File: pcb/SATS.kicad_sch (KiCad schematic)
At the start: 36 parts, among them J1 Raspberry_Pi_2_3, J10 SENSE, J11 SENSE Power, J12 EXT_GPIO, J13 EXT_GPIO, J14 EXT_GPIO, J2 A00-432-262-450, J3 AudioJack4_SwitchTR1, J4 5V, J5 3.3V, J6 Card LED, J7 Wiegand, J8 Beep, J9 Card Power, SW1 Main Door Switch, SW2 Serv Door Switch, SW3 Third Reed Switch, U1 MCP23017_SP, U2 MCP23017_SP, U3 CD40109BE, U4 IRLZ14PBF

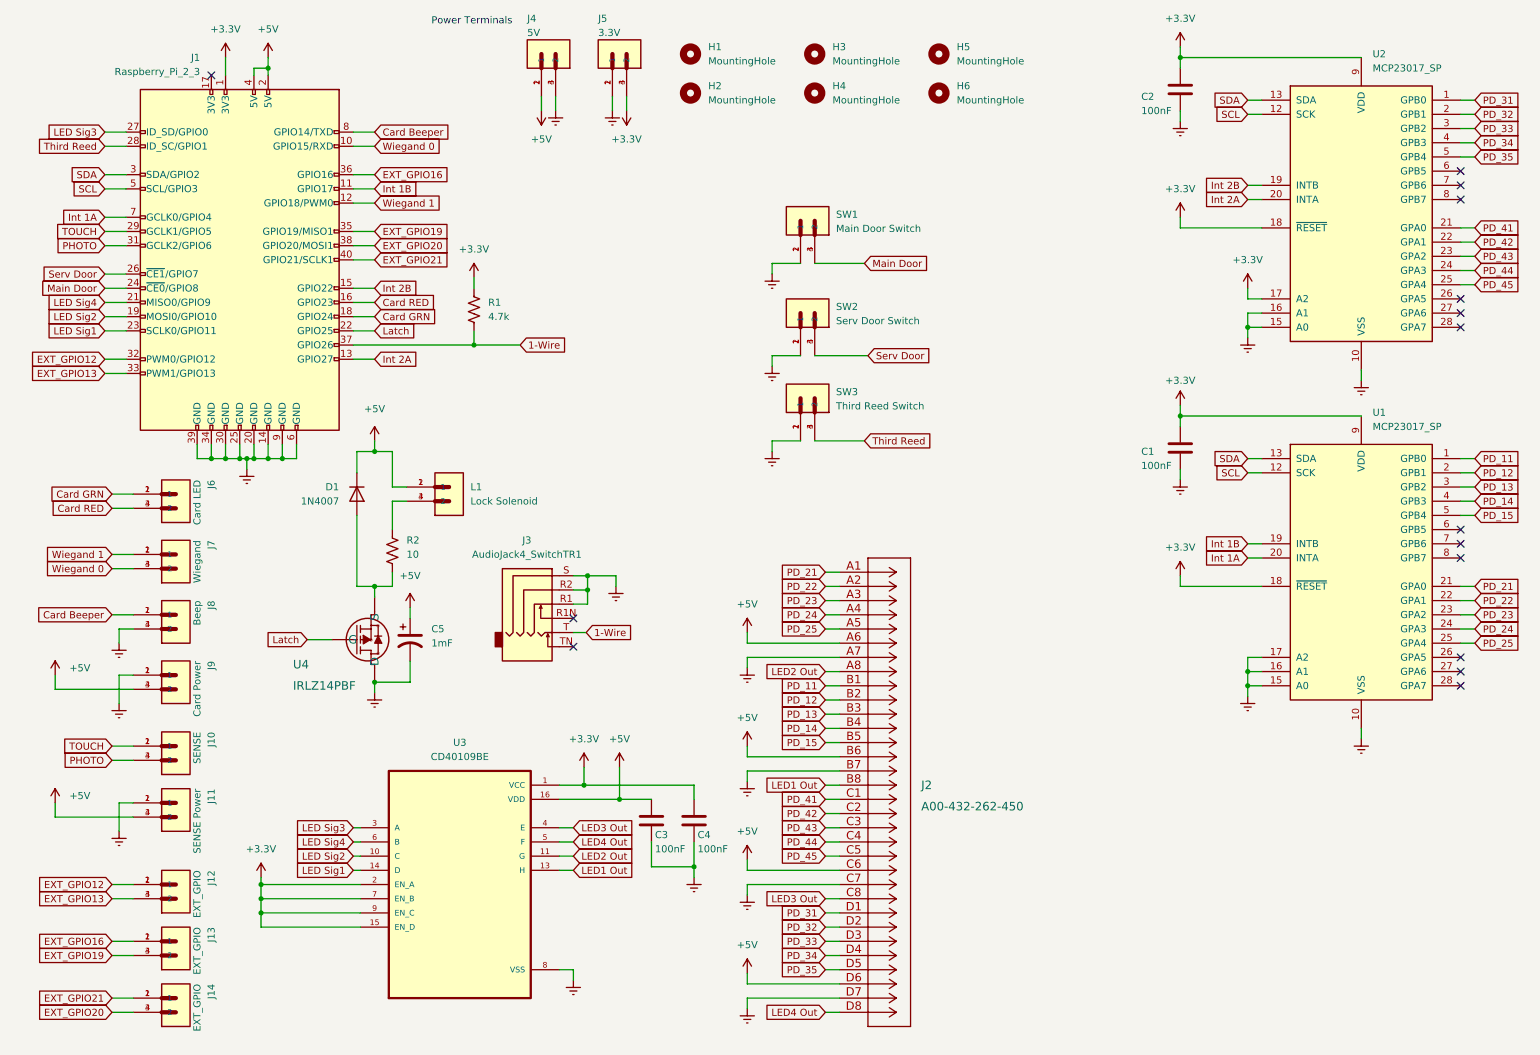
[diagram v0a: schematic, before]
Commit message: Rev 4 - Pretest
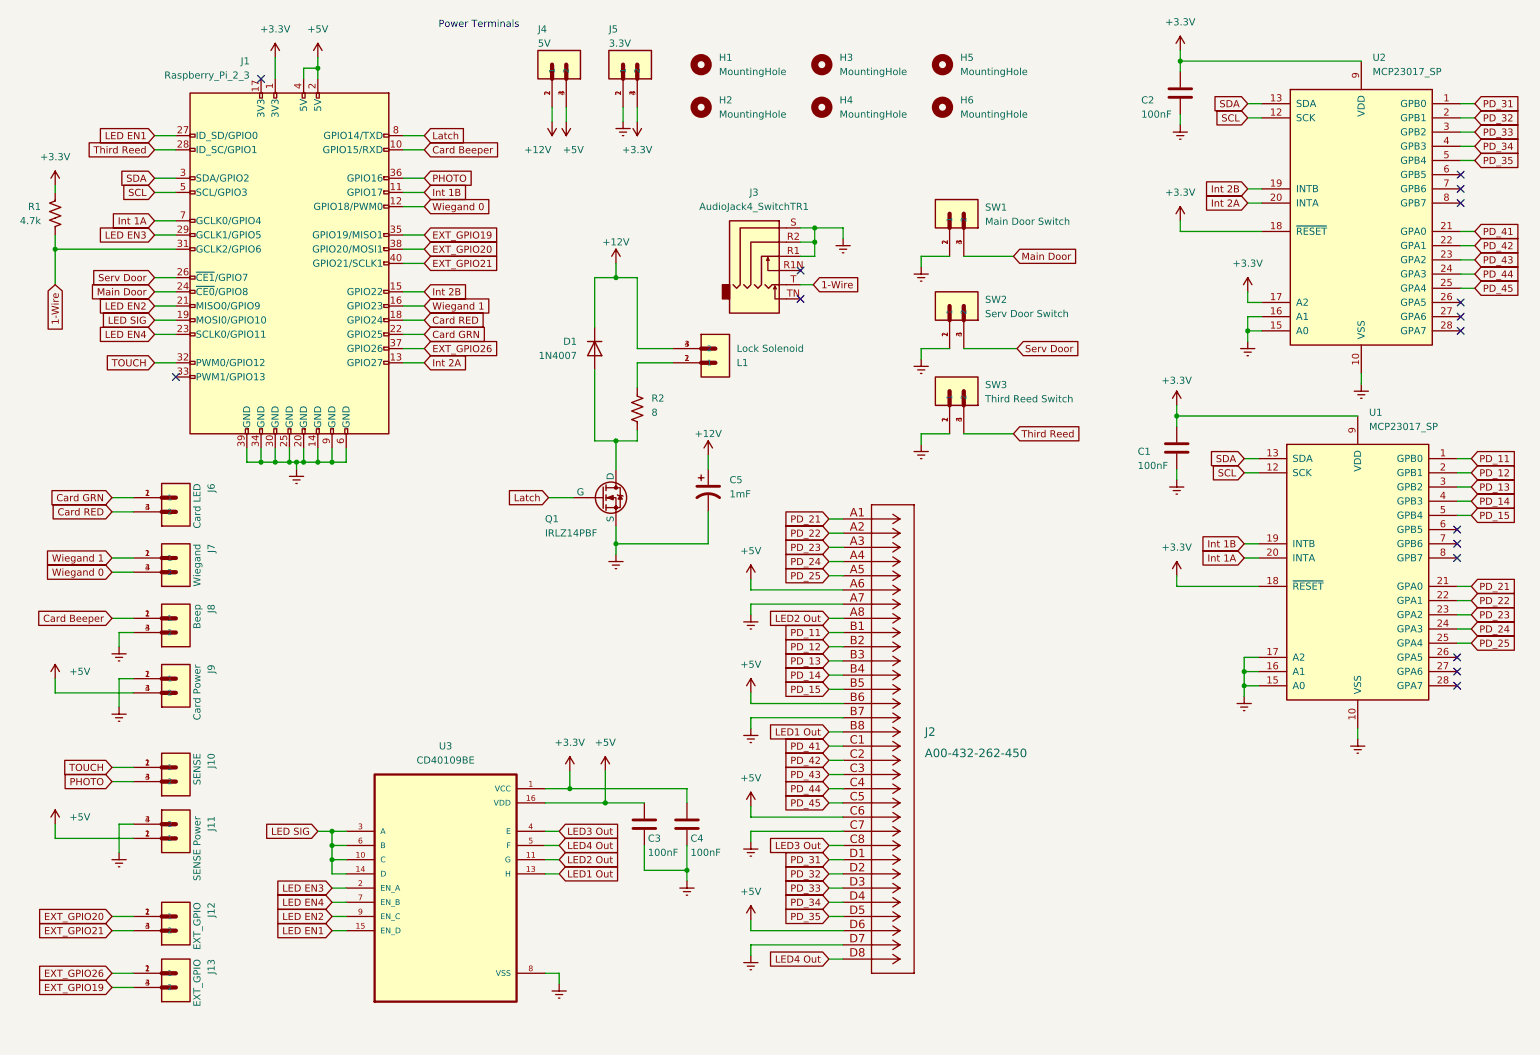
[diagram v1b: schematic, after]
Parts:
- removed J14: EXT_GPIO, TerminalConn:PHOENIX_1862042, symbol TerminalConn:1862042
- removed U4: IRLZ14PBF, Package_TO_SOT_THT:TO-220-3_Horizontal_TabDown, symbol IRLZ14PBF:IRLZ14PBF
- added Q1: IRLZ14PBF, Package_TO_SOT_THT:TO-220-3_Horizontal_TabDown, symbol Simulation_SPICE:NMOS
- R2: value 10 -> 8
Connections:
- net +3V3: no longer U3.15 (EN_D), U3.2 (EN_A), U3.7 (EN_B), U3.9 (EN_C)
- net +5V: now also J11.1, J11.2 (1), J4.3 (2), J4.4 (2); no longer C5.1, D1.1 (K), J11.3 (2), J11.4 (2), J4.1, J4.2 (1), L1.1, L1.2 (1)
- net 1-Wire: now also J1.31 (GCLK2/GPIO6); no longer J1.37 (GPIO26)
- net Card Beeper: now also J1.10 (GPIO15/RXD); no longer J1.8 (GPIO14/TXD)
- net Card GRN: now also J1.22 (GPIO25); no longer J1.18 (GPIO24)
- net Card RED: now also J1.18 (GPIO24); no longer J1.16 (GPIO23)
- net EXT_GPIO20: now also J12.1, J12.2 (1)
- net EXT_GPIO21: now also J12.3 (2), J12.4 (2)
- net Earth: now also J11.3 (2), J11.4 (2), Q1.3 (S); no longer J11.1, J11.2 (1), J4.3 (2), J4.4 (2)
- net Latch: now also J1.8 (GPIO14/TXD), Q1.2 (G); no longer J1.22 (GPIO25)
- net PHOTO: now also J1.36 (GPIO16); no longer J1.31 (GCLK2/GPIO6)
- net TOUCH: now also J1.32 (PWM0/GPIO12); no longer J1.29 (GCLK1/GPIO5)
- net Wiegand 0: now also J1.12 (GPIO18/PWM0); no longer J1.10 (GPIO15/RXD)
- net Wiegand 1: now also J1.16 (GPIO23); no longer J1.12 (GPIO18/PWM0)
- net at D1.2 (A), R2.2: now also Q1.1 (D)
- net +12V: now reaches L1.3 (2), L1.4 (2)
- net +12V: now also C5.1, D1.1 (K), J4.1, J4.2 (1); no longer R2.1
- removed net EXT_GPIO12: J1.32 (PWM0/GPIO12), J12.1, J12.2 (1)
- removed net EXT_GPIO13: J1.33 (PWM1/GPIO13), J12.3 (2), J12.4 (2)
- net EXT_GPIO16 renamed EXT_GPIO26
- net EXT_GPIO26: now also J1.37 (GPIO26); no longer J1.36 (GPIO16)
- net LED Sig1 renamed LED EN4
- net LED EN4: now also U3.7 (EN_B); no longer U3.14 (D)
- net LED Sig2 renamed LED SIG
- net LED SIG: now also U3.14 (D), U3.3 (A), U3.6 (B)
- net LED Sig3 renamed LED EN1
- net LED EN1: now also U3.15 (EN_D); no longer U3.3 (A)
- net LED Sig4 renamed LED EN2
- net LED EN2: now also U3.9 (EN_C); no longer U3.6 (B)
- new net: L1.1, L1.2 (1), R2.1
- new net LED EN3: J1.29 (GCLK1/GPIO5), U3.2 (EN_A)
- no-connect marks 15 -> 16
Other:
- moved on the sheet: C1, C2, C3, C4, C5, D1, H1, H2, H3, H4, H5, H6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
